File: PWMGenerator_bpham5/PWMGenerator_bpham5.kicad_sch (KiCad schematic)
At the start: 29 parts, among them J1 Conn_01x03, Q1 2N3904, Q2 2N3904, Q3 2N3906, Q4 2N3906, SW1 SW_SPST, U1 LM7805_TO220, U2 LM339

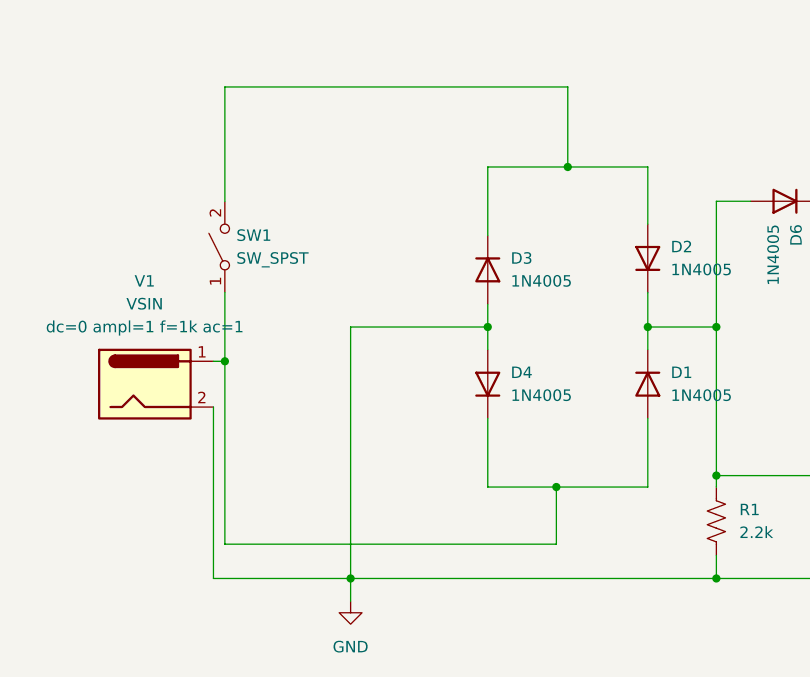
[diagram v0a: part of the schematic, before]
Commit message: part b fixed
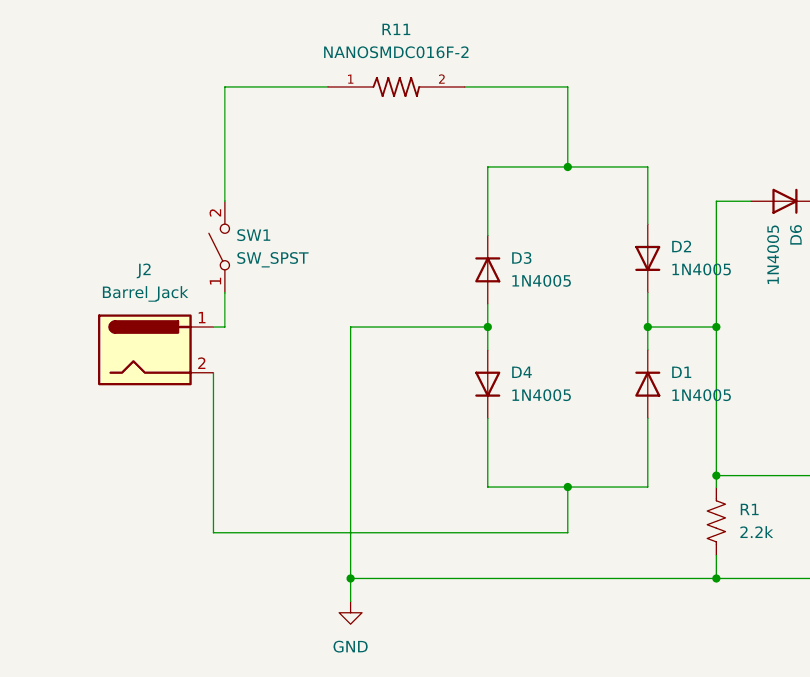
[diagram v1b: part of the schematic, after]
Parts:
- removed V1: VSIN, Connector_BarrelJack:BarrelJack_CUI_PJ-063AH_Horizontal, symbol Connector:Barrel_Jack
- added J2: Barrel_Jack, Connector_BarrelJack:BarrelJack_CUI_PJ-063AH_Horizontal, symbol Connector:Barrel_Jack
- added R11: NANOSMDC016F-2, NANOSMDC016F-2:RESC3115X65N, symbol NANOSMDC016F-2:NANOSMDC016F-2
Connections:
- net at D1.2 (A), D4.1 (K): now also J2.2; no longer SW1.1 (A)
- net at D2.2 (A), D3.1 (K): now also R11.2; no longer SW1.2 (B)
- new net: J2.1, SW1.1 (A)
- new net: R11.1, SW1.2 (B)
